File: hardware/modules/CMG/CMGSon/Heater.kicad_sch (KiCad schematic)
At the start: 36 parts, among them J301 HeaterLiPo, J302 THR1, J303 THR2, J304 Heater, J305 THR3, Q301 NMOS, U301 INA226, U302 MCP3424x-xSL, U904 MCP1501-20xSN

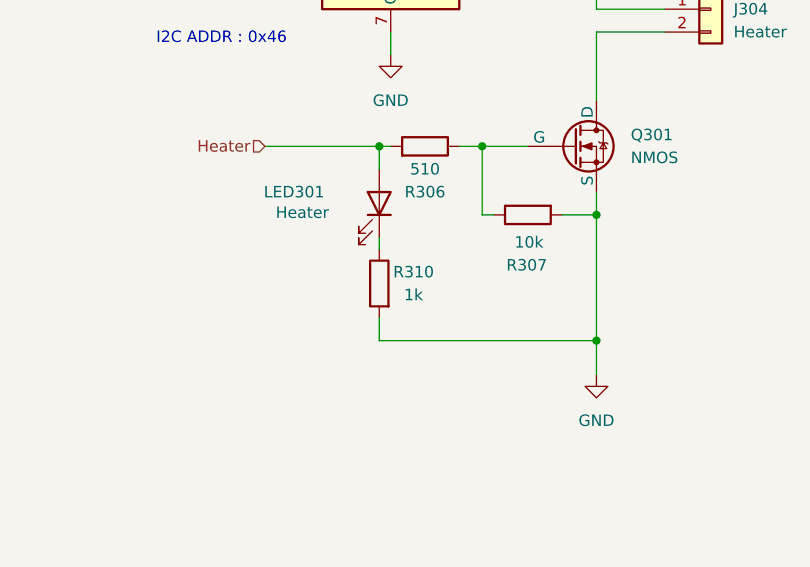
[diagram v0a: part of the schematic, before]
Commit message: LogicBoard一旦完成
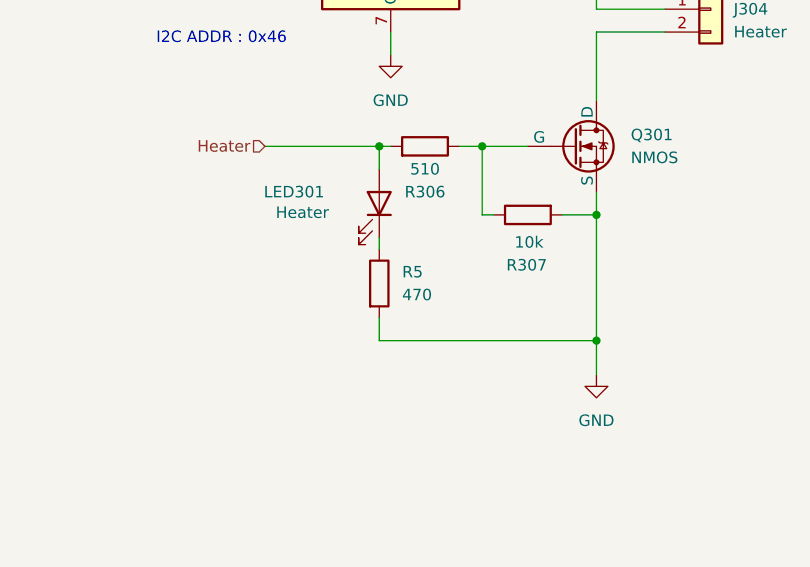
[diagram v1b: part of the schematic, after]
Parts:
- removed R310: 1k, Resistor_SMD:R_0402_1005Metric, symbol Device:R
- added R5: 470, Resistor_SMD:R_0402_1005Metric, symbol Device:R
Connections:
- net GND: now also R5.2
- net at LED301.1 (K): now also R5.1
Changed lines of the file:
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@@
-	(symbol
-		(lib_id "Device:R")
-		(at 212.09 123.19 0)
-		(mirror y)
-		(unit 1)
-		(exclude_from_sim no)
-		(in_bom yes)
-		(on_board yes)
-		(dnp no)
-		(property "Reference" "R310"
-			(at 215.9 121.92 0)
-			(effects
-				(font
-					(size 1.27 1.27)
-				)
-			)
-		)
-		(property "Value" "1k"
-			(at 215.9 124.46 0)
-			(effects
-				(font
-					(size 1.27 1.27)
-				)
-			)
-		)
-		(property "Footprint" "Resistor_SMD:R_0402_1005Metric"
-			(at 213.868 123.19 90)
-			(effects
-				(font
-					(size 1.27 1.27)
-				)
-				(hide yes)
-			)
-		)
-		(property "Datasheet" "~"
-			(at 212.09 123.19 0)
-			(effects
-				(font
-					(size 1.27 1.27)
-				)
-				(hide yes)
-			)
-		)
-		(property "Description" "Resistor"
-			(at 212.09 123.19 0)
-			(effects
-				(font
-					(size 1.27 1.27)
-				)
-				(hide yes)
-			)
-		)
-		(property "LCSC" "C25123"
-			(at 212.09 123.19 0)
-			(effects
-				(font
-					(size 1.27 1.27)
-				)
-				(hide yes)
-			)
-		)
-		(pin "1"
-		)
-		(pin "2"
-		)
-		(instances
-			(project "Heater"
-				(path "/4eb245a9-6c21-4f00-ae42-6a498711dd85/c55431da-8938-47ef-8924-54f36b792cab"
-					(reference "R310")
-					(unit 1)
-				)
-			)
-			(project "Heater"
-				(path "/861a27ed-ba4b-4fa4-8155-a8d1929fc215"
-					(reference "R108")
-					(unit 1)
-				)
-			)
-		)
-	)
 	(symbol
 		(lib_id "Device:R")
@@
 					(unit 1)
 				)
+			)
+		)
+	)
+	(symbol
+		(lib_id "Device:R")
+		(at 212.09 123.19 0)
+		(unit 1)
+		(exclude_from_sim no)
+		(in_bom yes)
+		(on_board yes)
+		(dnp no)
+		(fields_autoplaced yes)
+		(property "Reference" "R5"
+			(at 214.63 121.92 0)
+			(effects
+				(font
+					(size 1.27 1.27)
+				)
+				(justify left)
+			)
+		)
+		(property "Value" "470"
+			(at 214.63 124.46 0)
+			(effects
+				(font
+					(size 1.27 1.27)
+				)
+				(justify left)
+			)
+		)
+		(property "Footprint" "Resistor_SMD:R_0402_1005Metric"
+			(at 210.312 123.19 90)
+			(effects
+				(font
+					(size 1.27 1.27)
+				)
+				(hide yes)
+			)
+		)
+		(property "Datasheet" "~"
+			(at 212.09 123.19 0)
+			(effects
+				(font
+					(size 1.27 1.27)
+				)
+				(hide yes)
+			)
+		)
+		(property "Description" ""
+			(at 212.09 123.19 0)
+			(effects
+				(font
+					(size 1.27 1.27)
+				)
+				(hide yes)
+			)
+		)
+		(property "LCSC" "C25117"
+			(at 212.09 123.19 0)
+			(effects
+				(font
+					(size 1.27 1.27)
+				)
+				(hide yes)
+			)
+		)
+		(pin "1"
+		)
+		(pin "2"
+		)
+		(instances
+			(project "CMGSon"
+				(path "/4eb245a9-6c21-4f00-ae42-6a498711dd85/c55431da-8938-47ef-8924-54f36b792cab"
+					(reference "R5")
+					(unit 1)
+				)
